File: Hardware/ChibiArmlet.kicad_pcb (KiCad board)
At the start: 2 copper layers, 8 x 8 mm, 62 parts, among them Q2 MMBT2222, Q3 LED_RGB 5050, SW1 BUTTON, SW2 BUTTON, SW3 BUTTON

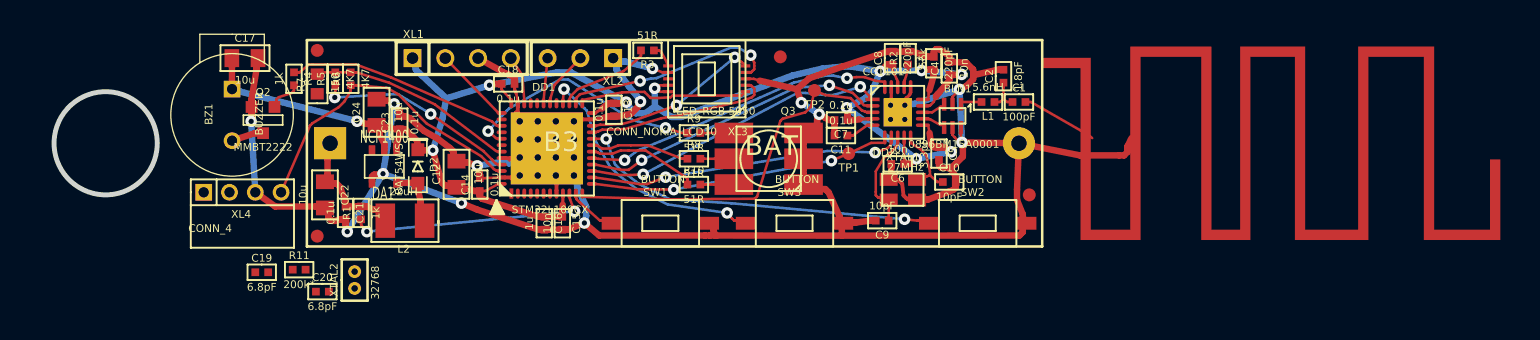
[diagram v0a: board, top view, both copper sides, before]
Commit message: Prototype sent to factory
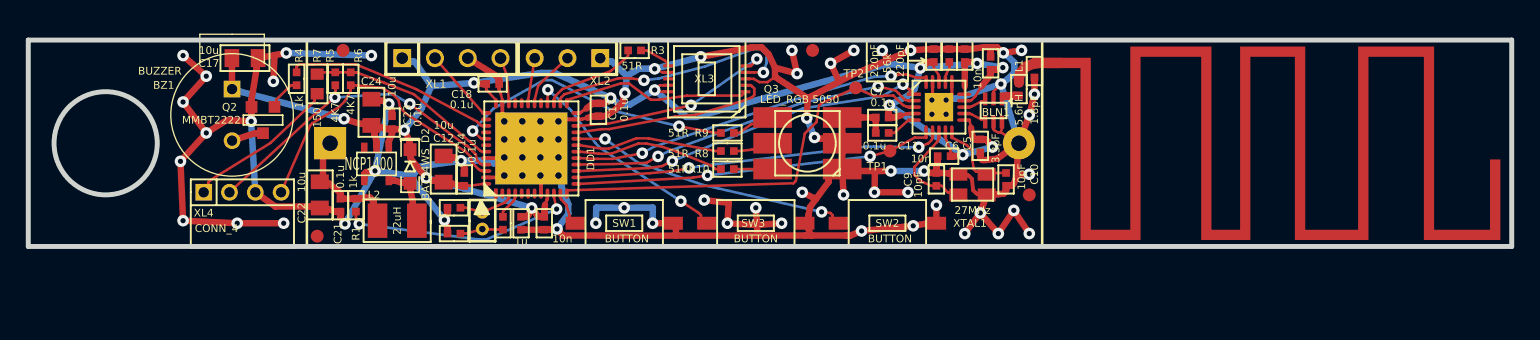
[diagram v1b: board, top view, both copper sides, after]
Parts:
- removed C1: 100pF, CAP_0402
- moved R11 16.2 mm to (195.8, 187.2), turned to 270 degrees
- moved C19 15.2 mm to (192.0, 188.0), turned to 180 degrees
- moved C20 12.1 mm to (192.0, 186.0), turned to 180 degrees
- moved XTAL2 10.9 mm to (194.2, 187.0)
- moved SW2 7.00 mm to (225.6, 187.2)
- moved XTAL1 5.41 mm to (232.2, 184.2)
- moved C9 5.28 mm to (229.4, 183.8), turned to 90 degrees
- moved C10 4.40 mm to (234.8, 183.8), turned to 270 degrees
- moved C6 3.65 mm to (230.0, 182.0)
- moved C5 3.26 mm to (232.8, 181.2)
- moved Q3 3.23 mm to (219.4, 181.0)
- moved DD2 3.22 mm to (229.6, 178.2)
- moved C4 3.22 mm to (233.6, 174.8)
- moved BLN1 3.21 mm to (233.8, 178.5)
- moved R2 3.21 mm to (230.4, 174.2)
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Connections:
- ANT1 pad 1: N-0000035 (its old number) -> N-0000010
- C2 pad 1: N-000009 (its old number) -> N-0000010
- L1 pad 1: N-000009 (its old number) -> N-0000010
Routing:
- net GND: track 223.3 -> 302.4 mm, vias 13 -> 56
- net /PeriphPwr1: track 0.00 -> 11.9 mm
- net /P_SCL: track 15.7 -> 25.7 mm
- net N-0000035 (its old number): track 6.70 -> 0.00 mm
- net /BTN2: track 28.4 -> 21.9 mm
- net N-0000031: track 0.00 -> 4.45 mm
- net N-0000010: track 0.00 -> 4.32 mm
- net /CC_GDO0: track 23.6 -> 27.9 mm
- net /CC_CS: track 24.2 -> 28.5 mm
- net /CC_MOSI: track 24.6 -> 28.5 mm
- net /CC_SCK: track 24.0 -> 27.8 mm
- net /RED_LED: track 7.71 -> 11.5 mm
- net /CC_MISO: track 23.8 -> 27.5 mm
- net /CC_GDO2: track 29.0 -> 32.6 mm
- net /GREEN_LED: track 19.1 -> 22.6 mm
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- added copper zone on B.Cu, net GND
- added copper zone on F.Cu, net GND
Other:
- board size 8 x 8 mm -> 115 x 16 mm
